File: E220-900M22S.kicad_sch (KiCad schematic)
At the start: 1 part, among them U3 E220-900M22S

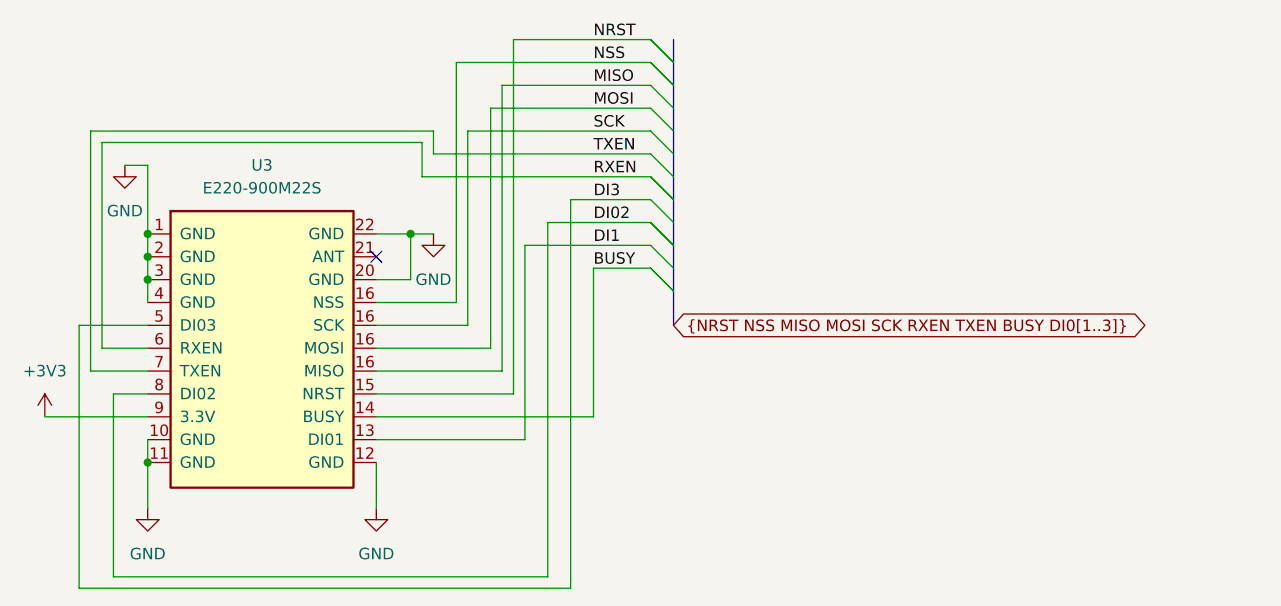
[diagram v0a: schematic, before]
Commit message: some cleanup. About to split two lra module branches.
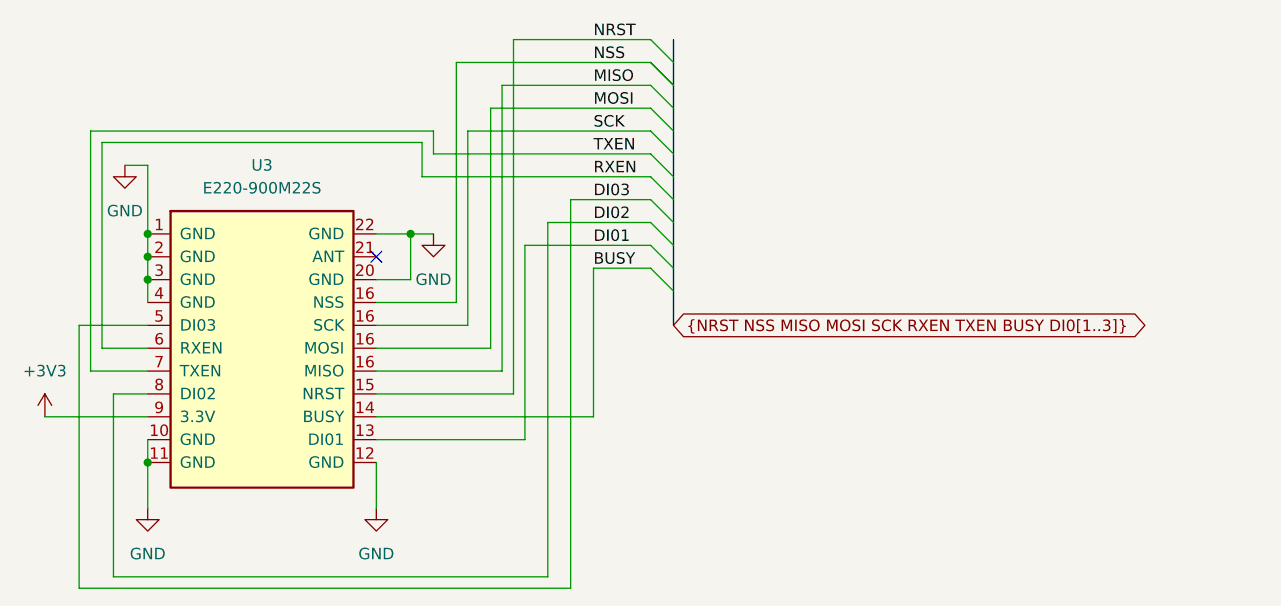
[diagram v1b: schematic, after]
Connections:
- net DI1 renamed DI01
- net DI3 renamed DI03
